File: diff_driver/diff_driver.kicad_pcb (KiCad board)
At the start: 2 copper layers, 32 x 22 mm, 14 parts, among them J1 CONN_01X07, J2 RJ45_LED, U1 am26ls31, U2 HT75XX-1

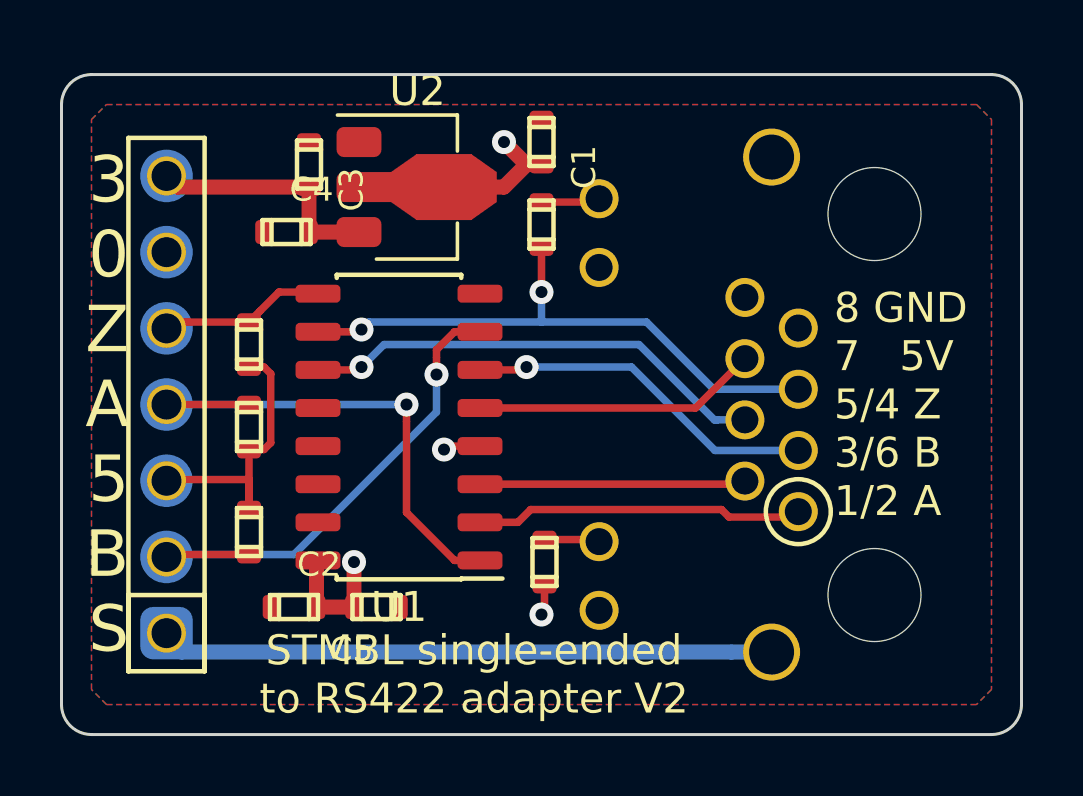
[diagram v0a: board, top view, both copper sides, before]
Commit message: hw
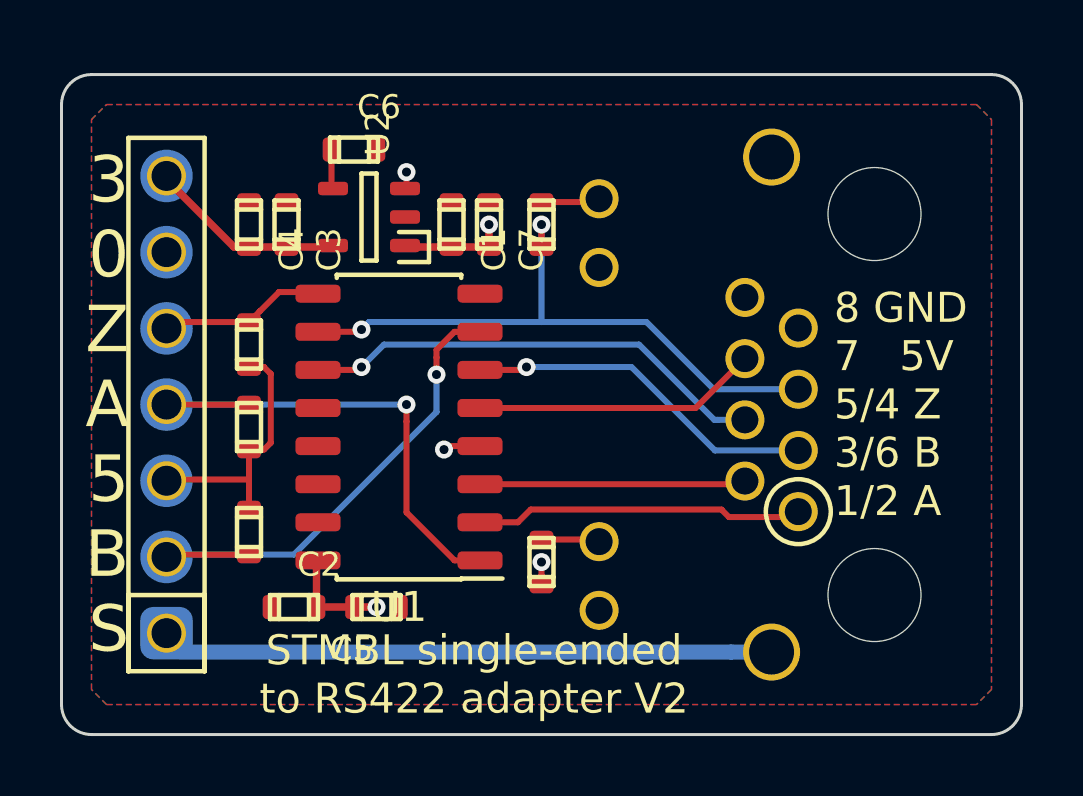
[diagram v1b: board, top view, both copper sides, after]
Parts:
- added C6: 100n, stmbl:C_0603, F.Cu at (152.8, 82.5)
- added C7: 1u, stmbl:C_0603, F.Cu at (157.2, 85.0)
- C4, C5: value 1n -> 1u
- U2: value HT75XX-1 -> LDO; footprint stmbl:SOT-89-3 -> stmbl:SOT-23-5
- moved C1 4.07 mm to (156.0, 85.0)
- moved C3 2.14 mm to (150.5, 85.0)
- moved U2 1.54 mm to (153.2, 84.8), turned to 180 degrees
- moved C4 1.27 mm to (149.2, 85.0), turned to 90 degrees
- moved R4 0.10 mm to (159.0, 96.2)
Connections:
- U2 pad 1: GND -> +5V
- U2 pad 2: +5V -> GND
- U2 pad 3: +3V3 -> +5V
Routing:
- net +5V: track 24.2 -> 19.5 mm, vias 4 -> 5
- net Net-(J2-Pad5): track 19.6 -> 21.1 mm
- net +3V3: track 8.07 -> 6.62 mm
- net Net-(C6-Pad2): track 0.00 -> 1.32 mm
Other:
- net class Default: clearance 0.2 -> 0.15; trace_width 0.25 -> 0.2; via_dia 0.8 -> 0.6; via_drill 0.4 -> 0.3
- rule trace_clearance: 0.2 -> 0.15
- rule via_min_size: 0.4 -> 0.6
